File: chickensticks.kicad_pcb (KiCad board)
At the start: 4 copper layers, 42 x 100 mm, 102 parts, among them J1 Conn_01x05_Pin, J2 HRO_TYPE-C-31-M-12, J3 Conn_01x04, J4 Conn_01x06, J5 Conn_01x06, J6 Conn_01x04, J7 Conn_01x04, J8 S02-25200300, J9 SMA, Q1 Si2371EDS, Q2 DMG9926UDM, Q3 2N7002, SW1 SKRPANE010, SW2 EC11E18244AU, U1 USBLC6-2SC6, U2 STM32L433CCTx, U3 TJA1042T-3, U4 LR2021IMLTRT, U5 LP5907MFX-3.3, U6 MCP73831-2-MC, U7 BQ29700, Y1 25 MHz, Y2 TG2520SMN 32.0000M-MCGNNM0

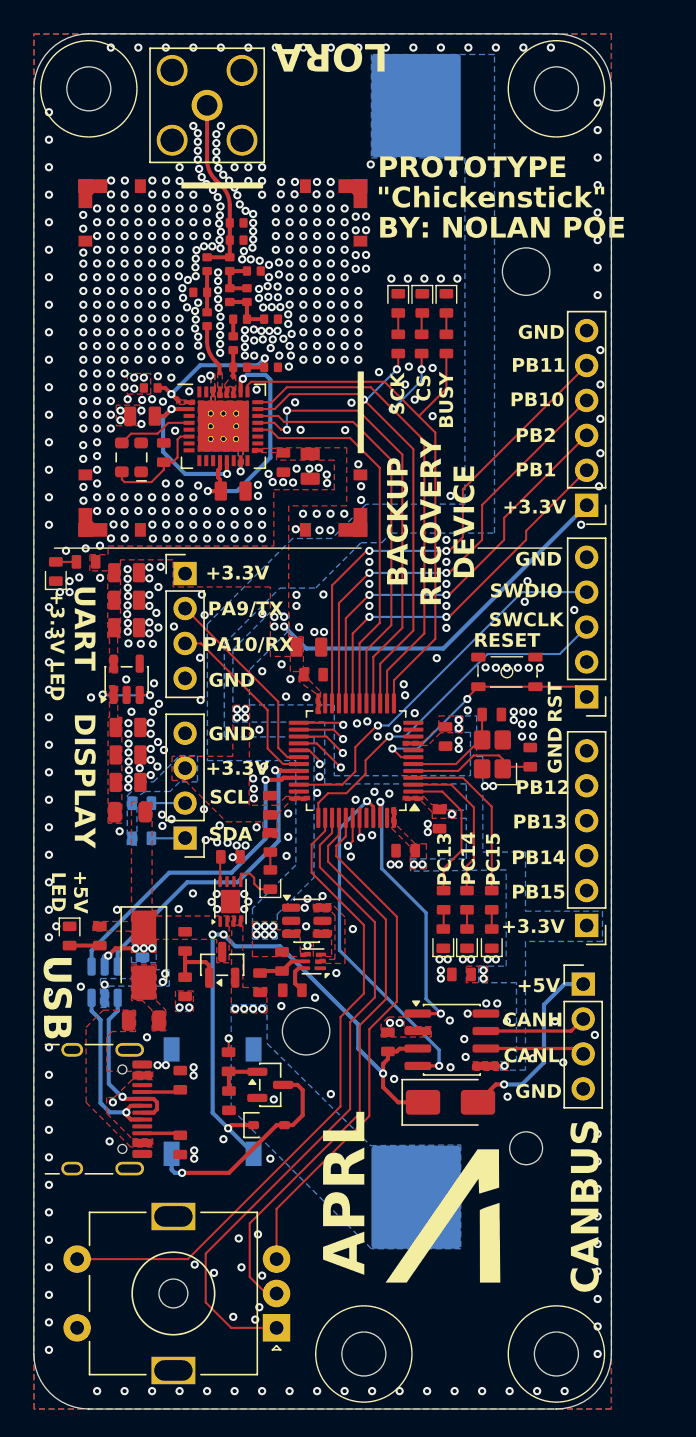
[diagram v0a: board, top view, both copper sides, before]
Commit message: Run cleanup tracks and vias
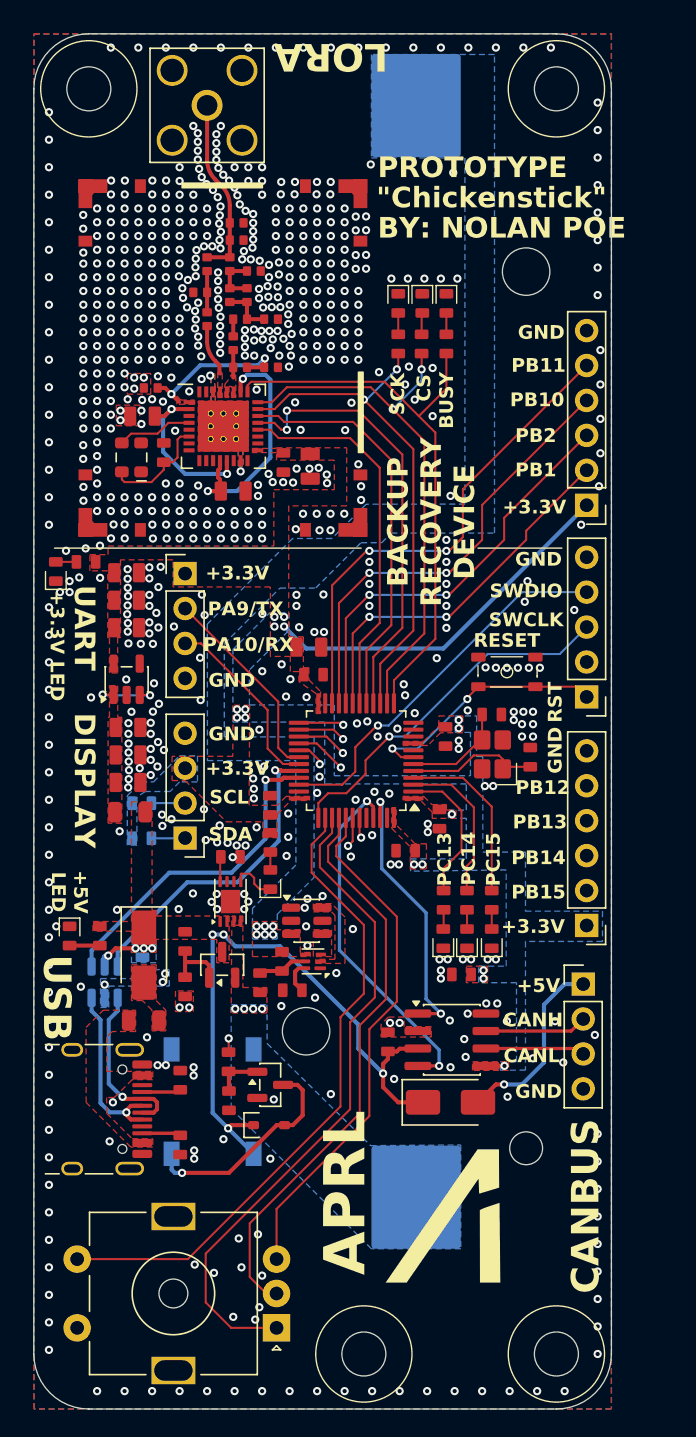
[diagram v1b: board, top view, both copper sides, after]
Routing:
- net /Microcontroller/~{RST}: track 18.1 -> 17.1 mm
- net +VUSB: track 48.5 -> 47.7 mm
- net /Microcontroller/ENC_C: track 42.0 -> 41.3 mm
- net /Microcontroller/CANL: track 7.24 -> 6.68 mm
- net Net-(J2-CC2): track 3.17 -> 2.62 mm
